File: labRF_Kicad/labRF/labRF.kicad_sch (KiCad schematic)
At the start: 41 parts, among them J1 select_rotary, J10 pwmC, J11 pwrIn, J2 mode_rotary, J3 lcd_socket, J4 comms, J5 si5351, J6 clk0, J7 clk2, J8 bias_pot, J9 pwmD, Q1 BC547, Q2 BC547, Q3 BC547, Q4 BC547, U1 ATmega328-P, U2 TL431LP, U3 74HC04, U4 L7805, Y1 20Mhz

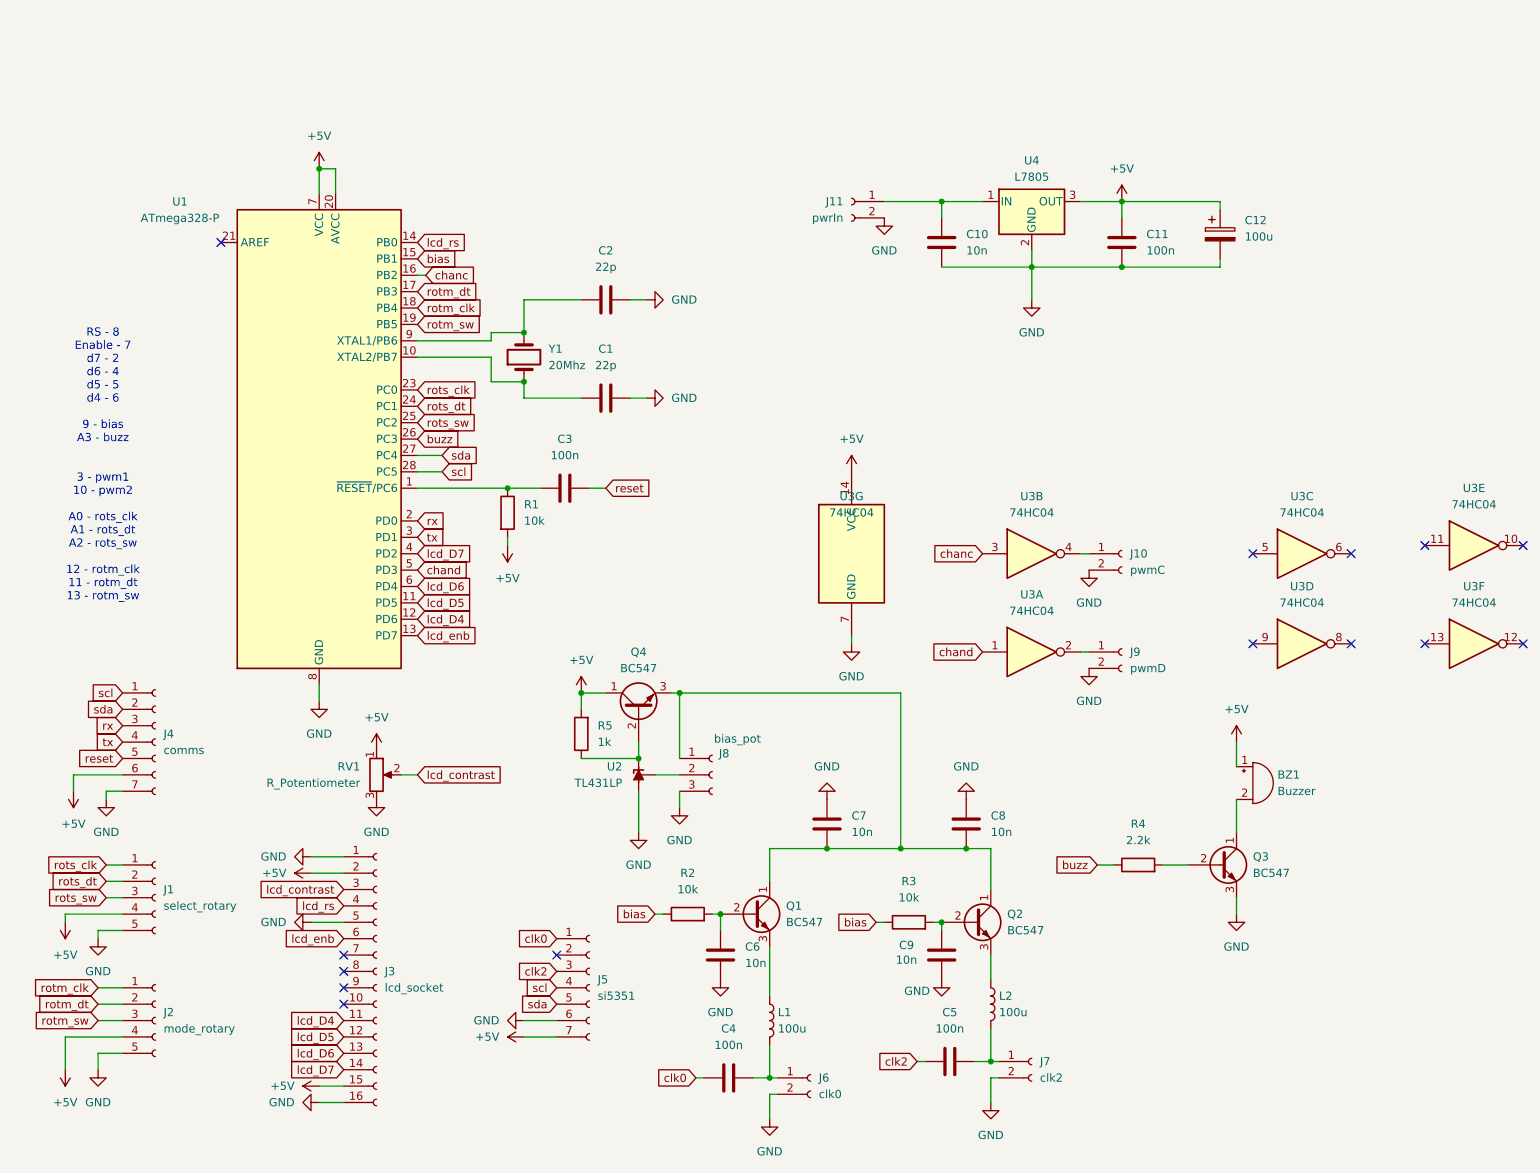
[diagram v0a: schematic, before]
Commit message: Finieshed PCB Design
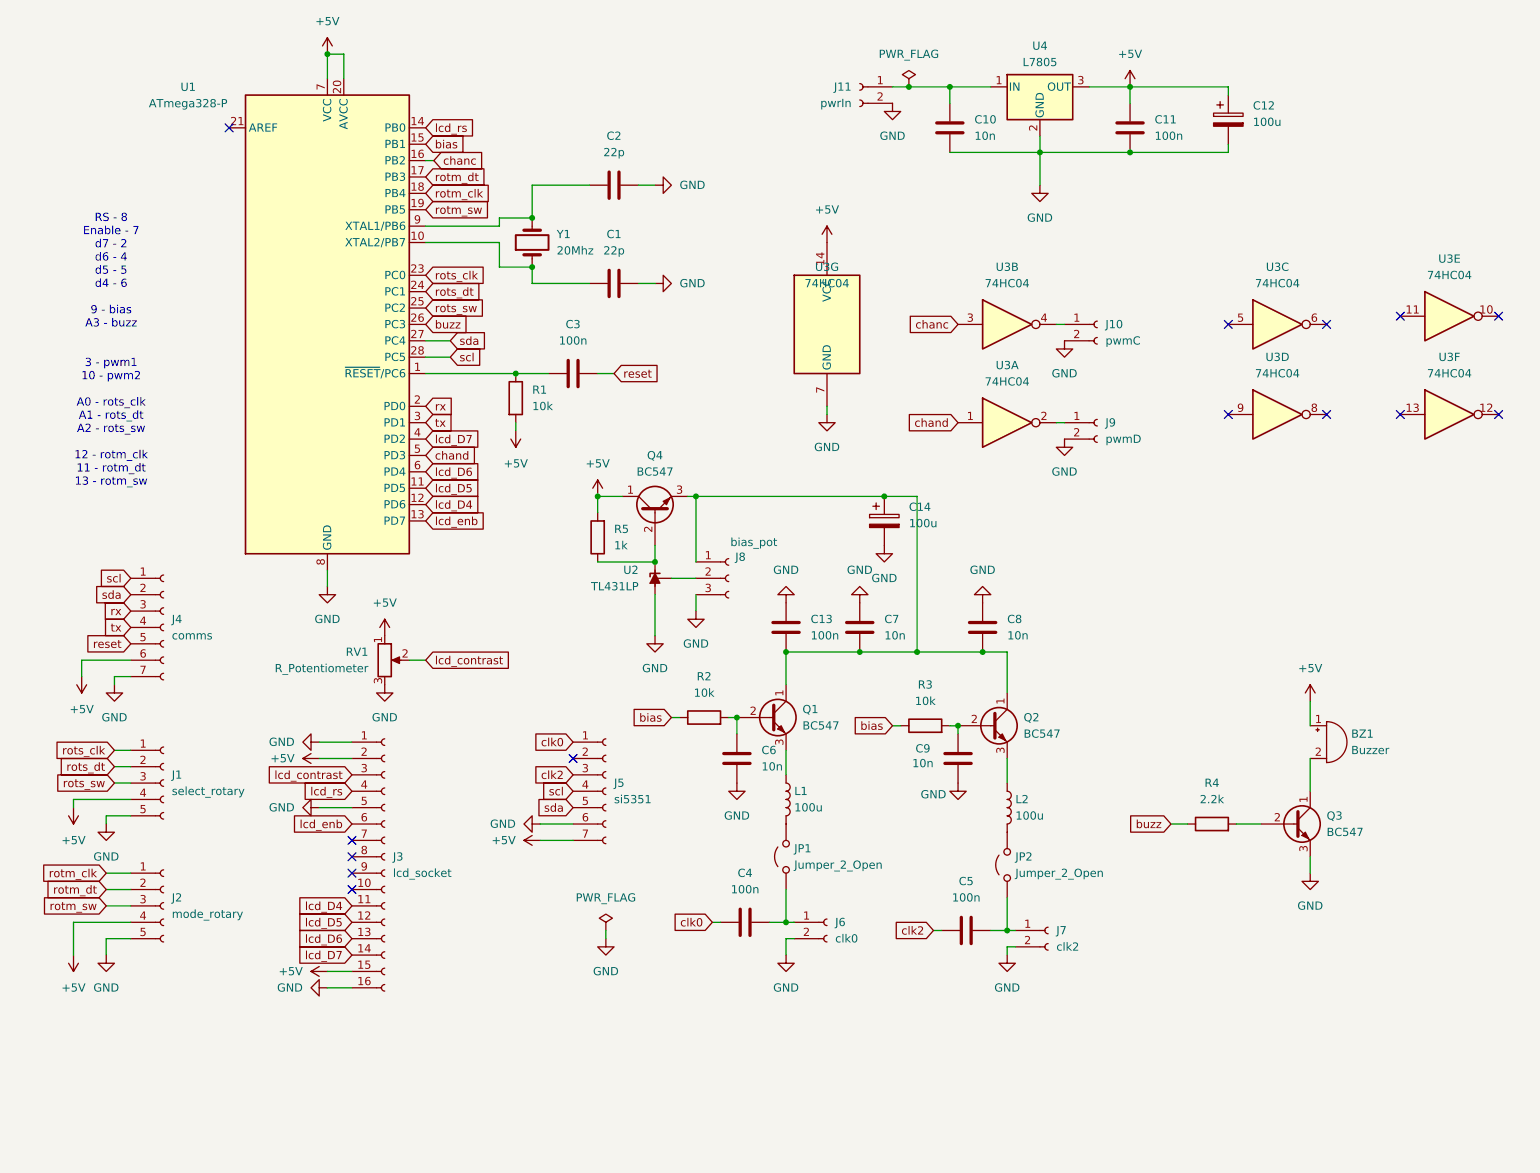
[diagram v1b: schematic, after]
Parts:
- added C13: 100n, Capacitor_THT:C_Disc_D5.0mm_W2.5mm_P2.50mm, symbol Device:C
- added C14: 100u, Capacitor_THT:CP_Radial_D8.0mm_P5.00mm, symbol Device:C_Polarized
- added JP1, JP2: Jumper_2_Open, Connector_PinHeader_2.54mm:PinHeader_1x02_P2.54mm_Vertical, symbol Jumper:Jumper_2_Open
- BZ1: footprint (none) -> Buzzer_Beeper:Buzzer_D14mm_H7mm_P10mm
- C1, C10, C11, C2, C3, C4, C5, C6, C7, C8, C9: footprint (none) -> Capacitor_THT:C_Disc_D5.0mm_W2.5mm_P2.50mm
- C12: footprint (none) -> Capacitor_THT:CP_Radial_D8.0mm_P5.00mm
- J1, J2: footprint (none) -> Connector_PinHeader_2.54mm:PinHeader_1x05_P2.54mm_Vertical
- J10, J11, J6, J7, J9: footprint (none) -> Connector_PinHeader_2.54mm:PinHeader_1x02_P2.54mm_Vertical
- J3: footprint (none) -> Connector_PinHeader_2.54mm:PinHeader_1x16_P2.54mm_Vertical
- J4, J5: footprint (none) -> Connector_PinHeader_2.54mm:PinHeader_1x07_P2.54mm_Vertical
- J8: footprint (none) -> Connector:FanPinHeader_1x03_P2.54mm_Vertical
- L1, L2: footprint (none) -> Inductor_THT:L_Toroid_Vertical_L14.7mm_W8.6mm_P5.58mm_Pulse_KM-1
- R1, R2, R3, R4, R5: footprint (none) -> Resistor_THT:R_Axial_DIN0207_L6.3mm_D2.5mm_P10.16mm_Horizontal
- RV1: footprint (none) -> Potentiometer_THT:Potentiometer_Bourns_3386P_Vertical
- U3: footprint (none) -> Package_DIP:DIP-14_W7.62mm
- U4: footprint (none) -> Package_TO_SOT_THT:TO-220-3_Vertical
- Y1: footprint (none) -> Crystal:Crystal_HC49-U_Vertical
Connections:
- net GND: now also C13.1, C14.2
- net at C7.2, C8.2, J8.1 (Pin_1)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: now also C13.2, C14.1
- net at C5.2, J7.1 (Pin_1): now also JP2.1 (A); no longer L2.2
- net at C4.2, J6.1 (Pin_1): now also JP1.1 (A); no longer L1.2
- new net: JP2.2 (B), L2.2
- new net: JP1.2 (B), L1.2
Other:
- moved on the sheet: BZ1, C1, C10, C11, C12, C2, C3, C4, C5, C6, C7, C8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
